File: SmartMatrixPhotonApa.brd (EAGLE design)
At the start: 40.6 x 35.6 mm, 13 parts, among them IC2 74AHC1G08DBV, IC3 74AHC1G08DBV, J1 0-DNP, U1 microSD

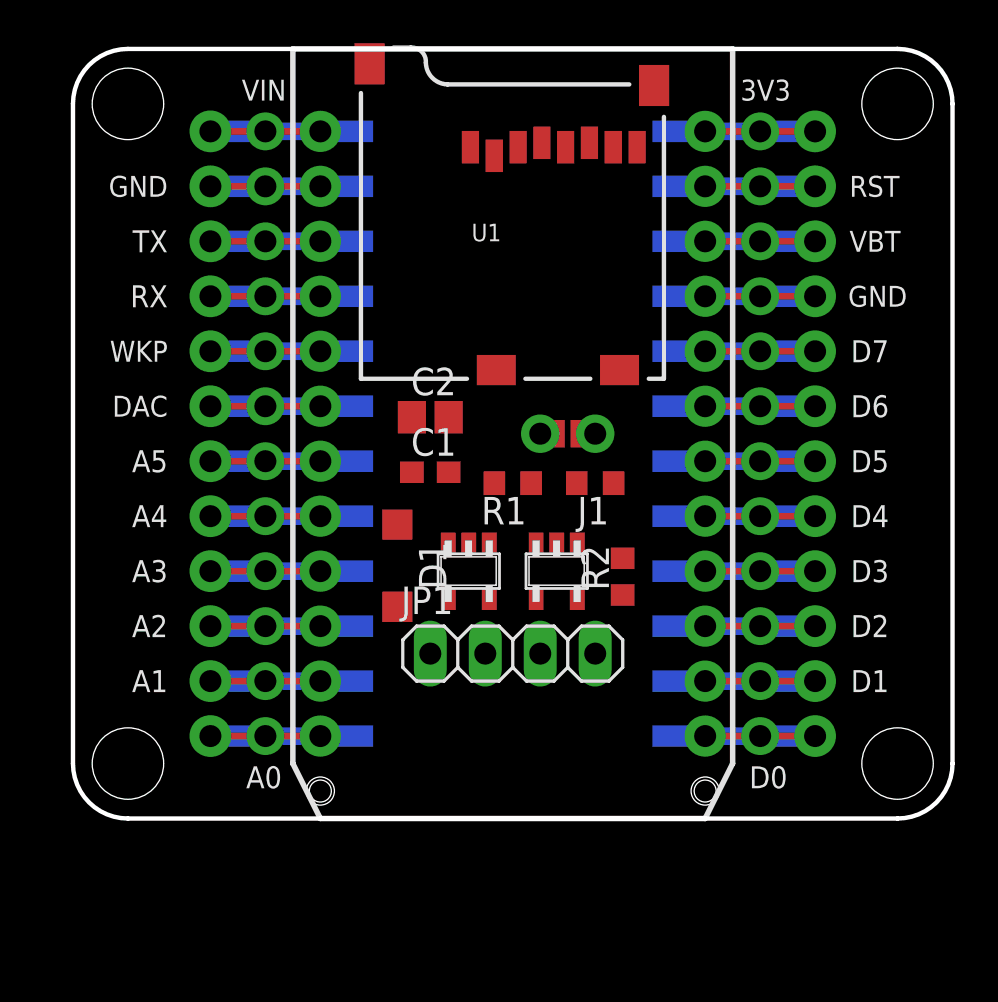
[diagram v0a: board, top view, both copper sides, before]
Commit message: Rough routing of board, not close to passing DRC
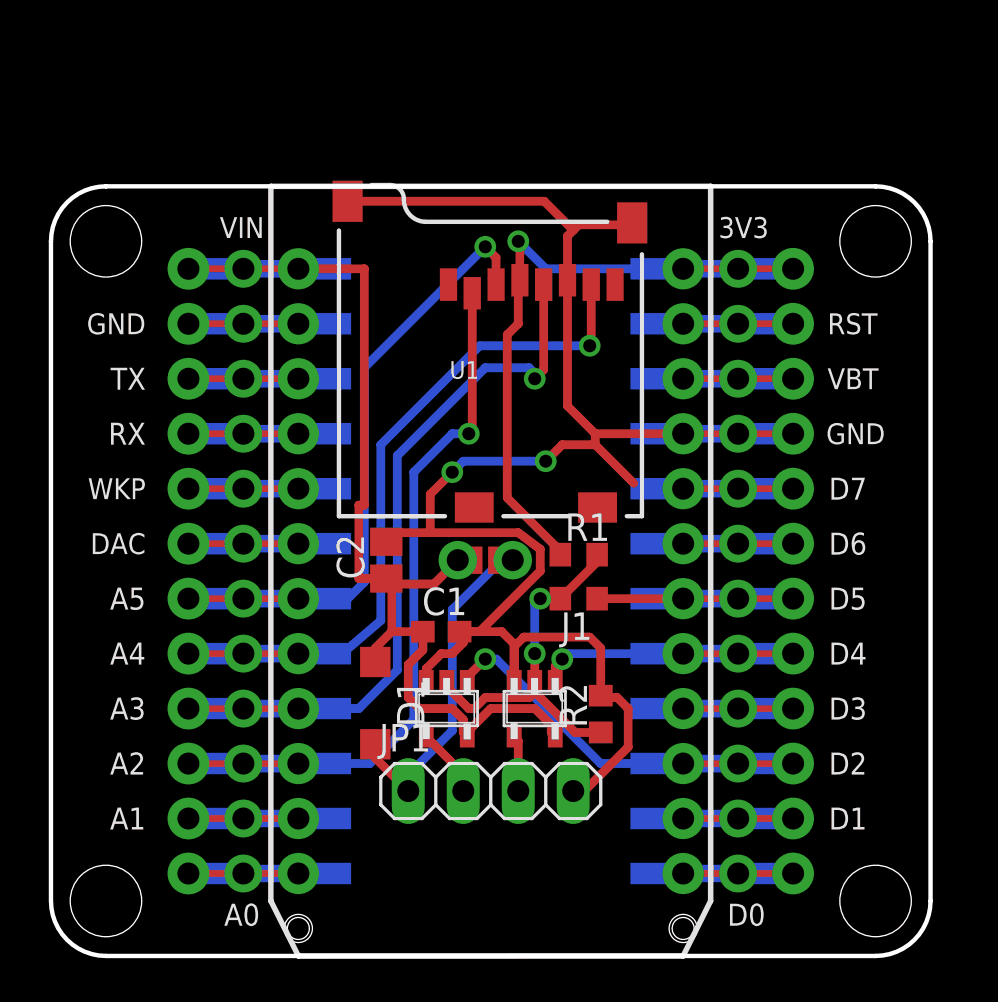
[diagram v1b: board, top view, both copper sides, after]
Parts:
- moved C1 7.38 mm to (18.3, 15.0)
- moved JP6 6.97 mm to (20.3, 18.3), turned to 180 degrees
- moved JP8 6.97 mm to (20.3, 18.3)
- moved C2 6.91 mm to (15.7, 18.3), turned to 90 degrees
- moved D1 6.43 mm to (15.2, 11.7)
- moved IC2 6.43 mm to (22.6, 11.4)
- moved IC3 6.43 mm to (18.5, 11.4)
- moved JP3 6.43 mm to (10.4, 0.00)
- moved R2 6.43 mm to (25.7, 11.2)
- moved U1 6.43 mm to (27.6, 20.3)
- moved JP1 6.43 mm to (20.6, 7.62)
- moved J1 5.39 mm to (24.6, 16.5)
- moved R1 4.49 mm to (24.6, 18.5), turned to 0 degrees
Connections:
- net V3.3 renamed 3V3
- new net N$1: JP3.GND@0, JP3.GND@0_1, JP3.GND@0_2, JP3.GND@0_S1, JP3.GND@0_S2
- net GND: now also JP3.GND@2, JP3.GND@2_1, JP3.GND@2_2, JP3.GND@2_S1, JP3.GND@2_S2; no longer JP3.GND@0, JP3.GND@0_1, JP3.GND@0_2, JP3.GND@0_S1, JP3.GND@0_S2
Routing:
- net GND: track 0.00 -> 77.4 mm, vias 0 -> 2
- net VIN: track 0.00 -> 45.6 mm
- net SPI_SCK: track 0.00 -> 26.6 mm, vias 0 -> 1
- net SD_CS: track 0.00 -> 25.9 mm, vias 0 -> 1
- net SPI_MISO: track 0.00 -> 25.4 mm, vias 0 -> 1
- net 3V3: track 0.00 -> 23.9 mm, vias 0 -> 1
- net SPI_MOSI: track 0.00 -> 21.6 mm, vias 0 -> 1
- net N$4: track 0.00 -> 17.0 mm, vias 0 -> 2
- net VEXT: track 0.00 -> 16.1 mm
- net LED_DAT: track 0.00 -> 12.5 mm, vias 0 -> 1
- net LED_CLK: track 0.00 -> 6.82 mm, vias 0 -> 1
- net LED_EN: track 0.00 -> 3.98 mm
- net N$3: track 0.00 -> 3.22 mm
- net N$2: track 0.00 -> 2.59 mm
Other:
- board text added: "Photon SMT Breakout Footprint originally by Particle"
- board text added: "Photon Shield Footprint originally by SparkFun, CC BY-SA 4.0"
- board text added: "Pixelmatix 2016 CC BY-SA 4.0"
- board text added: "Rev V3"
- board text added: "SmartMatrix APA Shield for Photon"

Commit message: Rev V0.1, ready to order prototypes
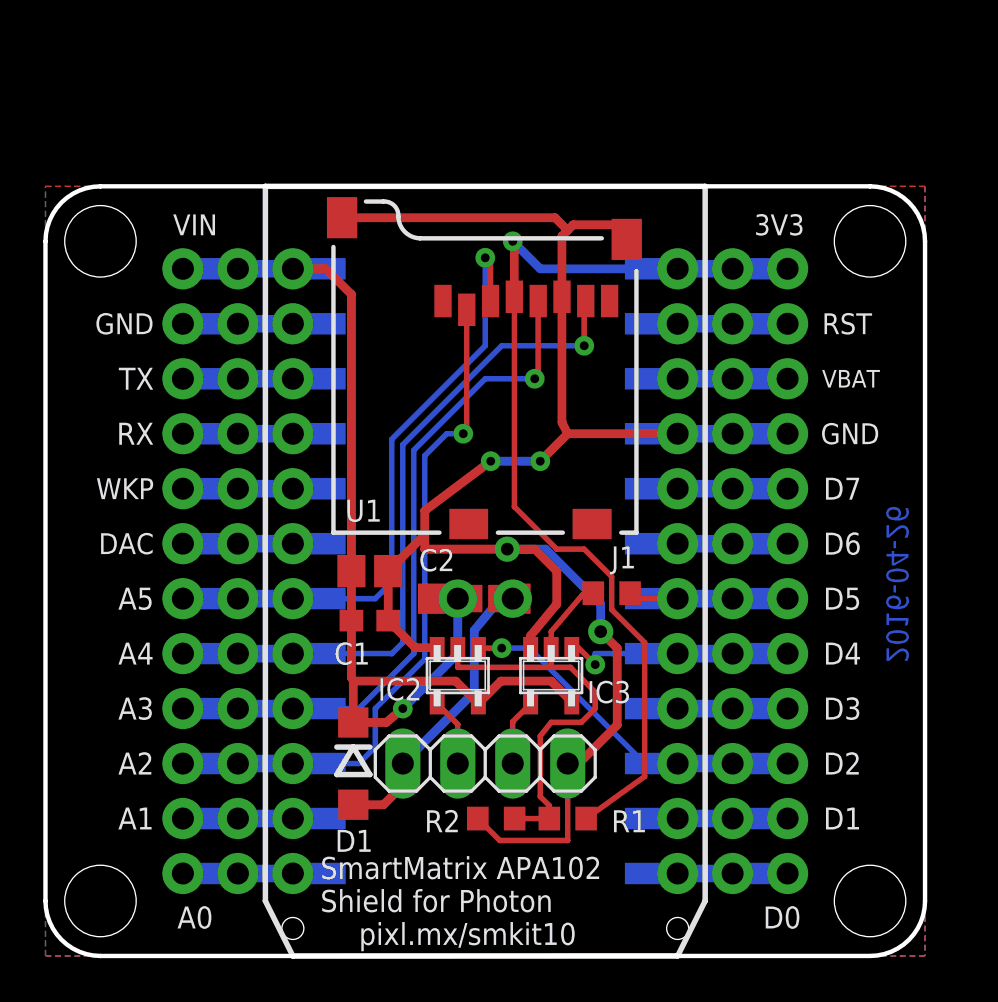
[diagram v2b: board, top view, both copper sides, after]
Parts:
- added D2: MBR0520LT, diode:SOD123
- moved R1 12.2 mm to (24.1, 6.35), turned to 180 degrees
- moved R2 6.82 mm to (20.8, 6.35), turned to 180 degrees
- moved C1 3.34 mm to (15.0, 15.5)
- moved D1 2.97 mm to (14.2, 8.89)
- moved JP6 1.78 mm to (20.3, 16.5)
- moved JP8 1.78 mm to (20.3, 16.5)
- moved IC2 1.70 mm to (23.4, 13.0)
- moved IC3 1.61 mm to (19.1, 13.0)
- moved J1 1.55 mm to (26.2, 16.8)
- moved JP1 1.30 mm to (20.3, 8.89)
- moved C2 0.92 mm to (15.0, 17.8), turned to 0 degrees
- moved U1 0.80 mm to (27.3, 19.6)
- moved JP3 0.25 mm to (10.2, 0.00)
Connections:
- net N$2 renamed CLK
- net N$3 renamed DAT
- removed net N$1: JP3.GND@0, JP3.GND@0_1, JP3.GND@0_2, JP3.GND@0_S1, JP3.GND@0_S2
- net VEXT: now also D2.C
- net VIN: now also D2.A
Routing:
- net 3V3: track 23.9 -> 44.6 mm
- net SPI_MOSI: track 21.6 -> 28.8 mm
- net SPI_MISO: track 25.4 -> 31.9 mm
- net VIN: track 45.6 -> 51.7 mm, vias 0 -> 1
- net SD_CS: track 25.9 -> 31.6 mm
- net GND: track 77.4 -> 82.8 mm, vias 2 -> 4
- net LED_EN: track 3.98 -> 9.13 mm
- net SPI_SCK: track 26.6 -> 31.7 mm
- net LED_CLK: track 6.82 -> 11.8 mm
- net N$4: track 17.0 -> 21.8 mm, vias 2 -> 0
- net LED_DAT: track 12.5 -> 16.5 mm
- net VEXT: track 16.1 -> 14.6 mm
- net CLK: track 2.59 -> 3.11 mm
- added copper zone on layer 1, net GND
- added copper zone on layer 16, net GND
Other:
- board text added: "+5V"
- board text added: "2016-04-26"
- board text added: "CLK"
- board text added: "DAT"
- board text added: "GND"
- board text added: "IC2"
- board text added: "IC3"
- board text added: "Rev V0.1"
- board text added: "SmartMatrix APA102 Shield for Photon"
- board text added: "VEXT"
- board text added: "VIN"
- board text added: "pixl.mx/smkit10"
- board text removed: "Rev V3"
- board text removed: "SmartMatrix APA Shield for Photon"
